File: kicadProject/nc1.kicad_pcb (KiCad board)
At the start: 2 copper layers, 68 parts, among them J1 Conn_01x02, J2 Conn_01x03, Q1 2N7002, Q2 2N7002, Q4 BD911, U1 NCP1034, U2 NE5534, U3 NE5534

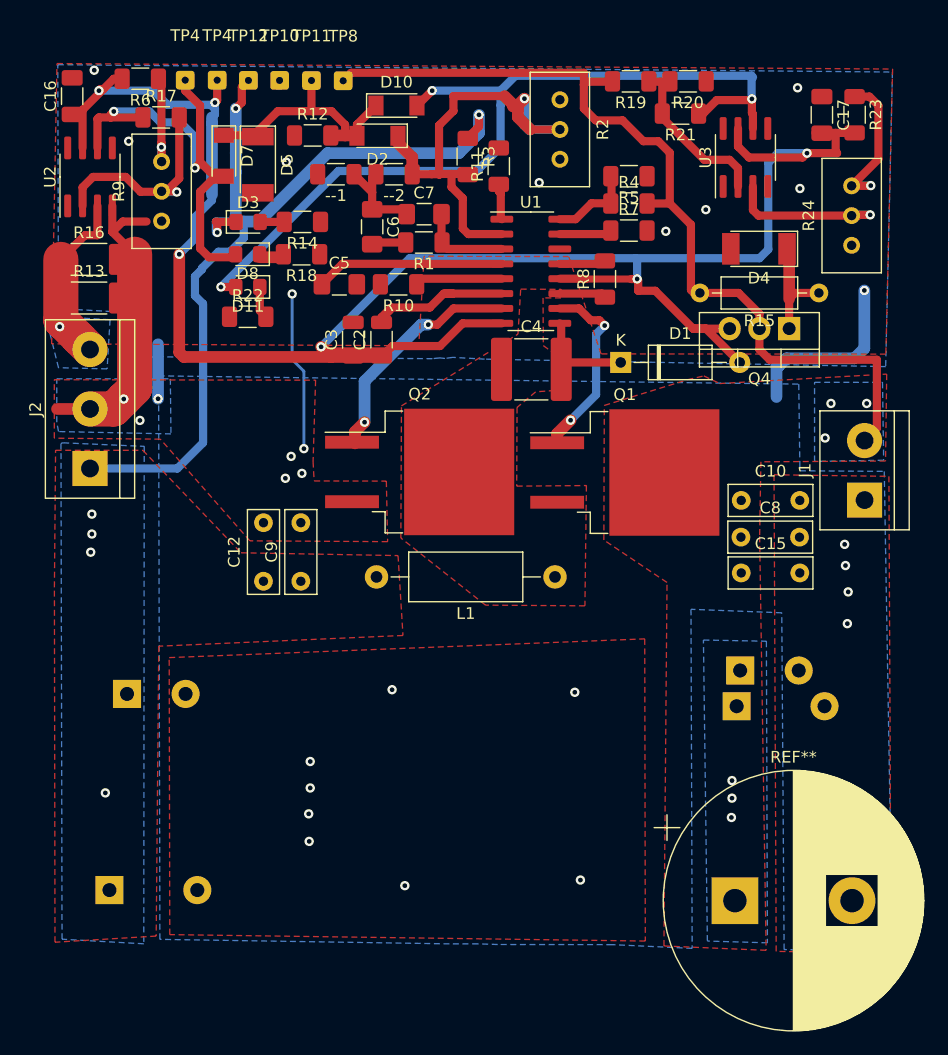
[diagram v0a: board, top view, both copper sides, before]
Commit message: more compensatioon
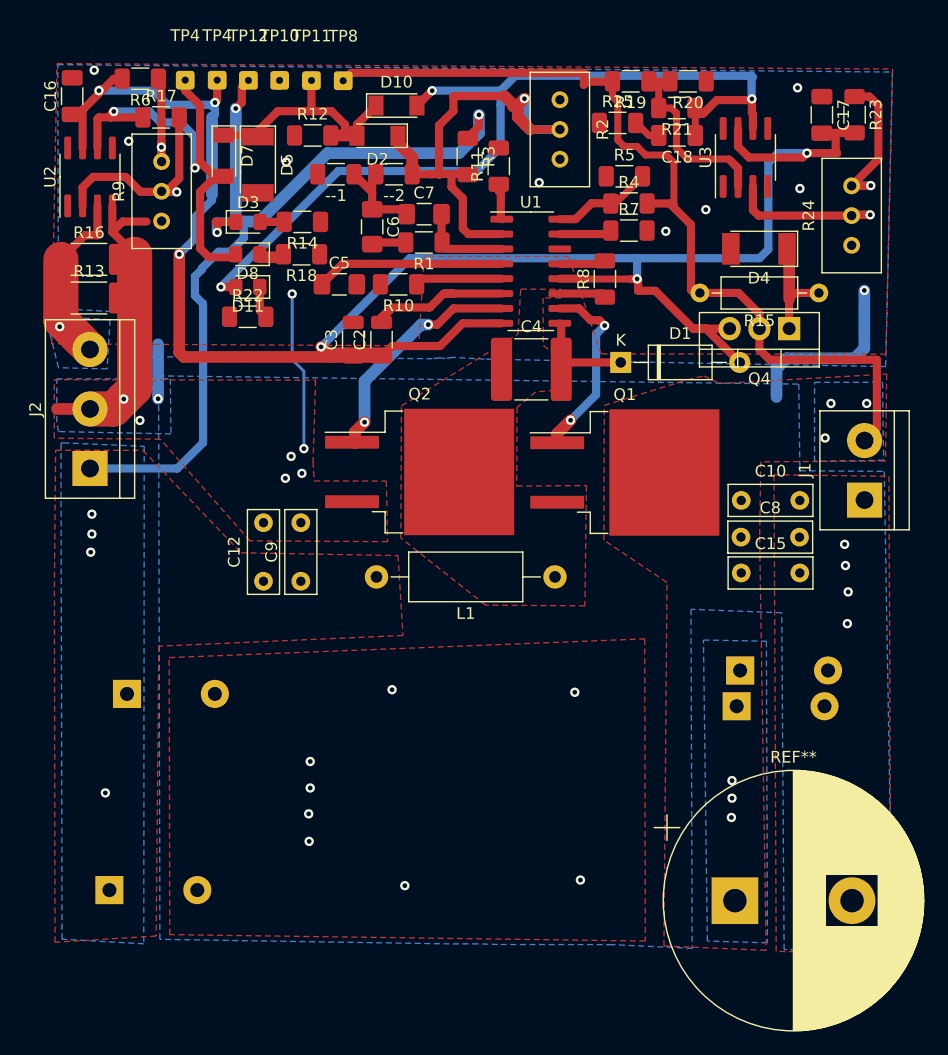
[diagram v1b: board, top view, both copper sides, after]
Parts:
- added C18: 470n, Capacitor_SMD:C_1206_3216Metric_Pad1.33x1.80mm_HandSolder, F.Cu at (71.7, 44.7)
- added R25: 4.7k, Resistor_SMD:R_1206_3216Metric_Pad1.30x1.75mm_HandSolder, F.Cu at (66.6, 43.6)
- C1: value C -> 100n; footprint Capacitor_THT:CP_Radial_D14.0mm_P5.00mm -> Capacitor_THT:CP_Radial_D18.0mm_P7.50mm
- C10: value C -> 100u
- C11, C8: value C -> 10u
- C12, C13: value C -> 100n
- C14: value C -> 100n; footprint Capacitor_THT:CP_Radial_D14.0mm_P5.00mm -> Capacitor_THT:CP_Radial_D16.0mm_P7.50mm
- C4: value 100nF -> 100nF 200V
- C5: value C -> 10n
- C9: value C -> 20u
- D1: value bav21 -> BAV21
- D11: value LED -> YELLOW
- D3: value LED -> GREEN
- D4: value D_Zener -> 15V
- D5: value D_Zener -> 5V
- D8: value LED -> RED
- L1: value INDUCTOR -> 100uH
- Q1, Q2: value 2N7002 -> AOB414
- R10, R8: value R -> 10k
- R11: value 4.7k -> 10k
- R13, R16: value R -> 0.27
- R15: value 5k -> 10k
- R18, R22: value 47k -> 470
- R19: value 10k -> 100k
- R2: value R_POT -> 20k
- R23: value 10k -> 0
- R24: value R_POT -> 100k
- R3: value R -> 47k
- R4: value 100k -> 220k
- R5: value 5k -> 12k
- R9: value R_POT -> 10k
- moved R21 0.56 mm to (71.7, 42.4)
- moved R5 0.39 mm to (67.2, 48.2), turned to 0 degrees
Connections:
- R2 pad 3: (no net) -> Net-(R2-Pad3)
- TP4 pad 1: Net-(D7-Pad2) -> 15V
- U2 pad 1: (no net) -> Net-(U2-Pad1)
- U2 pad 8: (no net) -> Net-(U2-Pad8)
- U3 pad 1: (no net) -> Net-(U3-Pad1)
- U3 pad 8: (no net) -> Net-(U3-Pad8)
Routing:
- net Net-(C18-Pad2): track 0.00 -> 2.49 mm
- net Net-(D9-Pad1): track 13.9 -> 16.4 mm
- net Net-(C18-Pad1): track 74.3 -> 76.7 mm
- net Net-(R4-Pad1): track 7.33 -> 8.67 mm
